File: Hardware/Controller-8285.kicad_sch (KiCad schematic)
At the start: 31 parts, among them J1 Conn_01x07_Male, J10 Conn_Coaxial, J2 Conn_01x04_Male, J3 Conn_01x02_Male, J4 Conn_01x02_Male, J5 Conn_01x02_Male, J6 Conn_01x02_Male, J7 Conn_01x08_Male, J8 QWIIC_Vertical, J9 QWIIC_Stackable, Q1 UMH3N, SW1 SW_Push, U1 ESP8285H16, Y1 26.000MHz

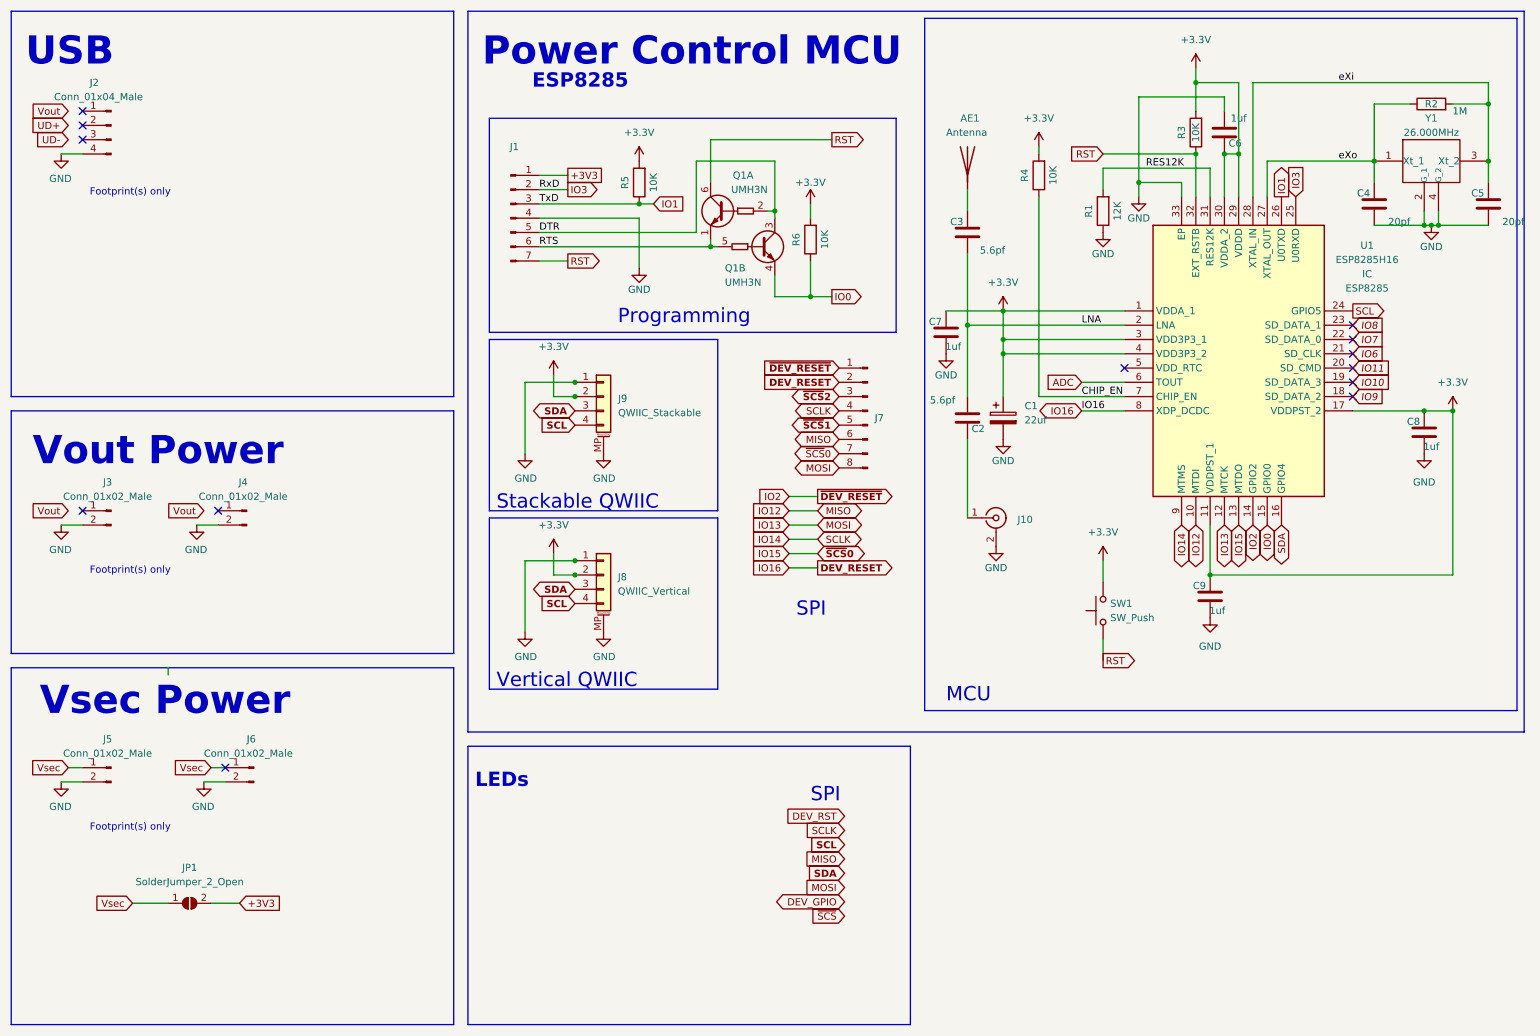
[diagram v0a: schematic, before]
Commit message: Working on the RP2040 & cleaning up stuff...
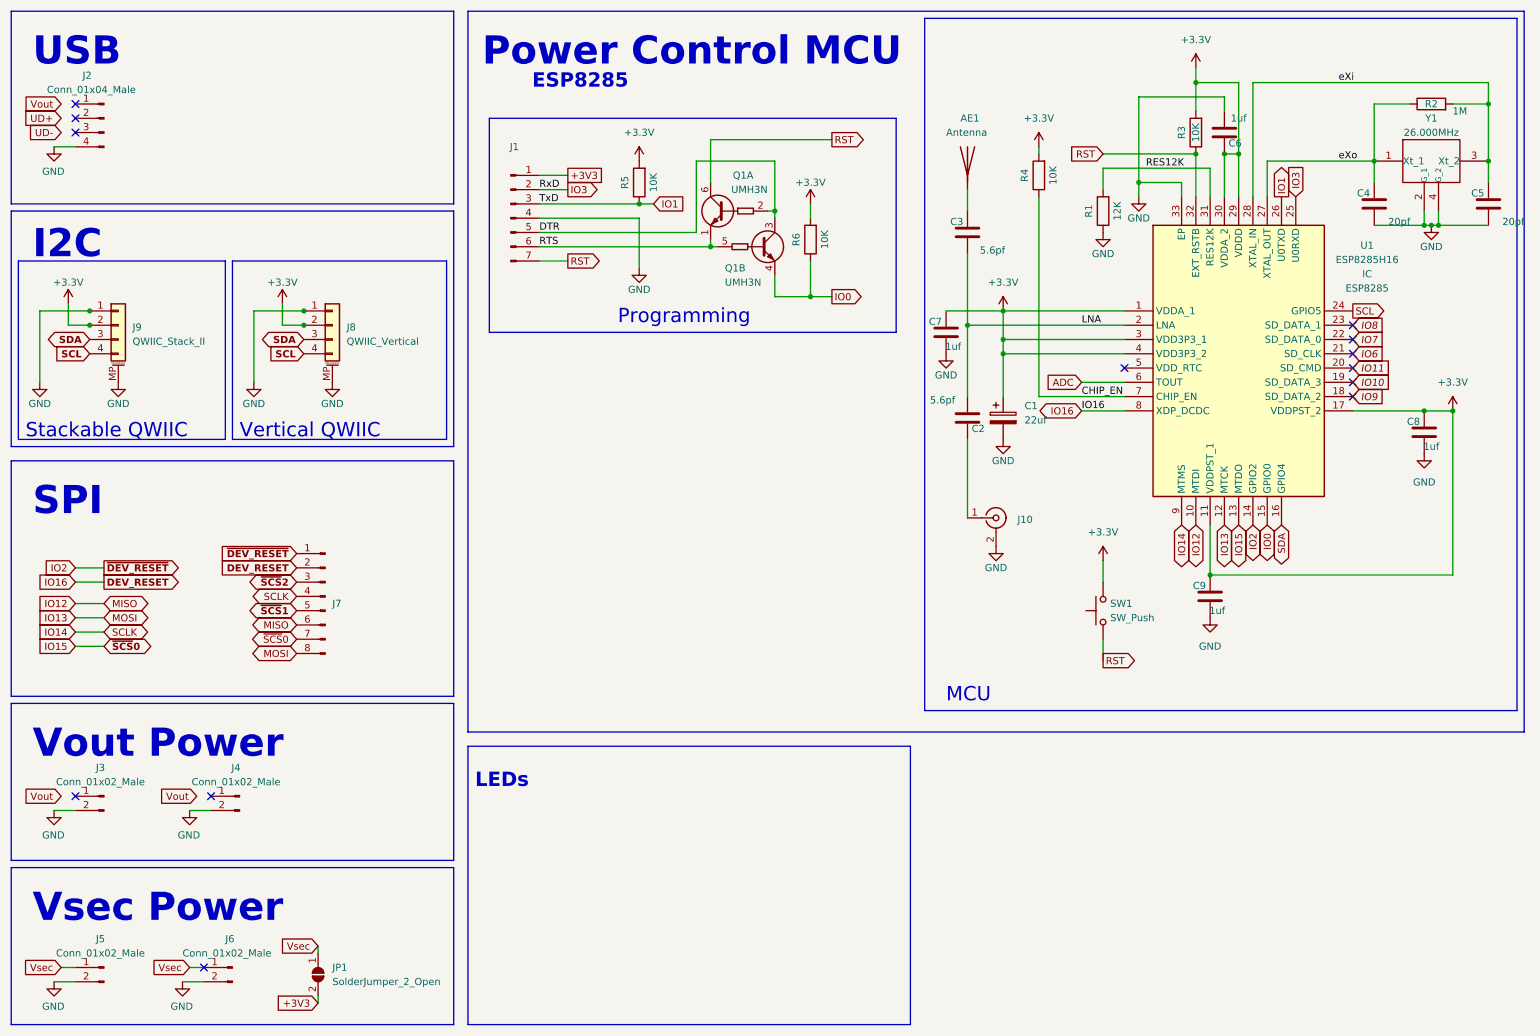
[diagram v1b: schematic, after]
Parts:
- J9: value QWIIC_Stackable -> QWIIC_Stack_II
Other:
- note added: "I2C"
- note removed: "Footprint(s) only"
- moved on the sheet: J2, J3, J4, J5, J6, J7, J8, J9, JP1
